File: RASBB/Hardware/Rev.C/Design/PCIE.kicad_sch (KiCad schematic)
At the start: 3 parts, among them J17 Conn_01x02_Pin, J4 X3157WS-98-9TV30

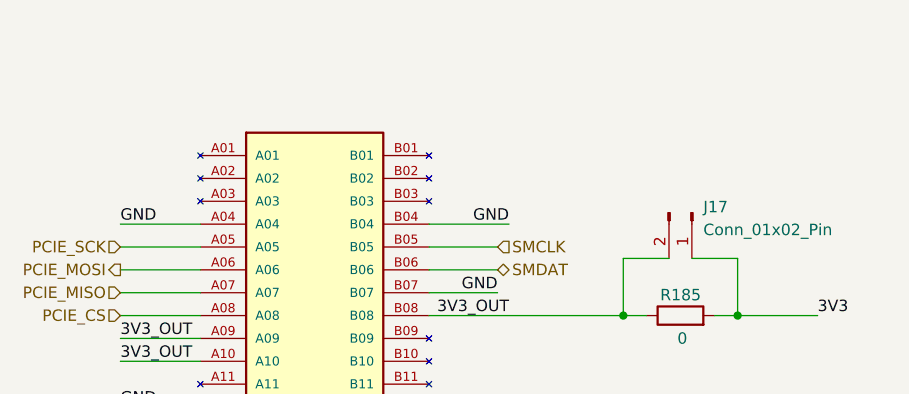
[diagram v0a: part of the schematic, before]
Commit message: Draft AC
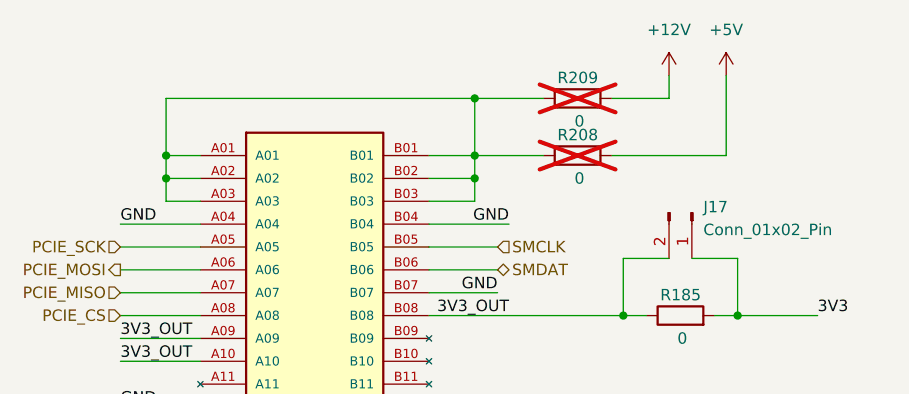
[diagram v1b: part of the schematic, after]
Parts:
- added R208, R209: 0, Resistor_SMD:R_1206_3216Metric, symbol Device:R
- J17: LCSC Part # (none) -> C492401; Mfr. Part # (none) -> PZ254V-11-02P
- J4: LCSC Part #  C5711253 -> (none)
- R185: Mfr. Part # (none) -> 1206W4F0000T5E
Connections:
- net +12V: now also R209.2
- net at J4.A01: now also J4.A02, J4.A03, J4.B01, J4.B02, J4.B03, R208.1, R209.1
- new net +5V: R208.2
